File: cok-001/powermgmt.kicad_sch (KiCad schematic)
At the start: 39 parts, among them J6004 +12V_MAIN, J6005 +5V_EVER, Q6001 FDQ7238AS, Q6002 FDQ7238AS, U6003 MB39A, U6008 NCP511SN18T1, U6011 NCP511, U6012 MM3141, U6014 MM1591, U6019 NCP511SN18T1, U6021 MM1591, U6022 MM1593

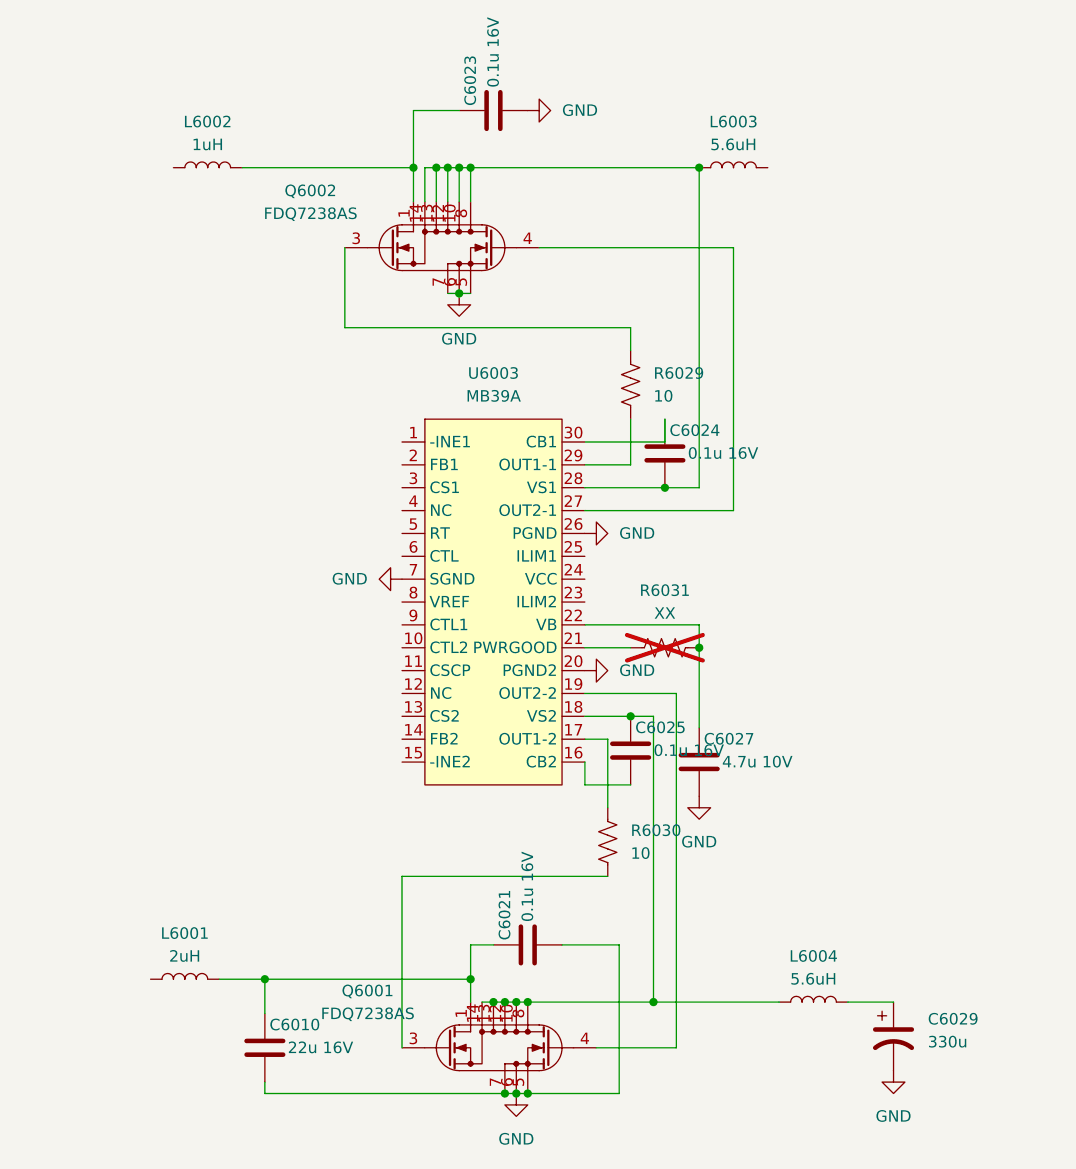
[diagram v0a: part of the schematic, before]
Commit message: update to 9
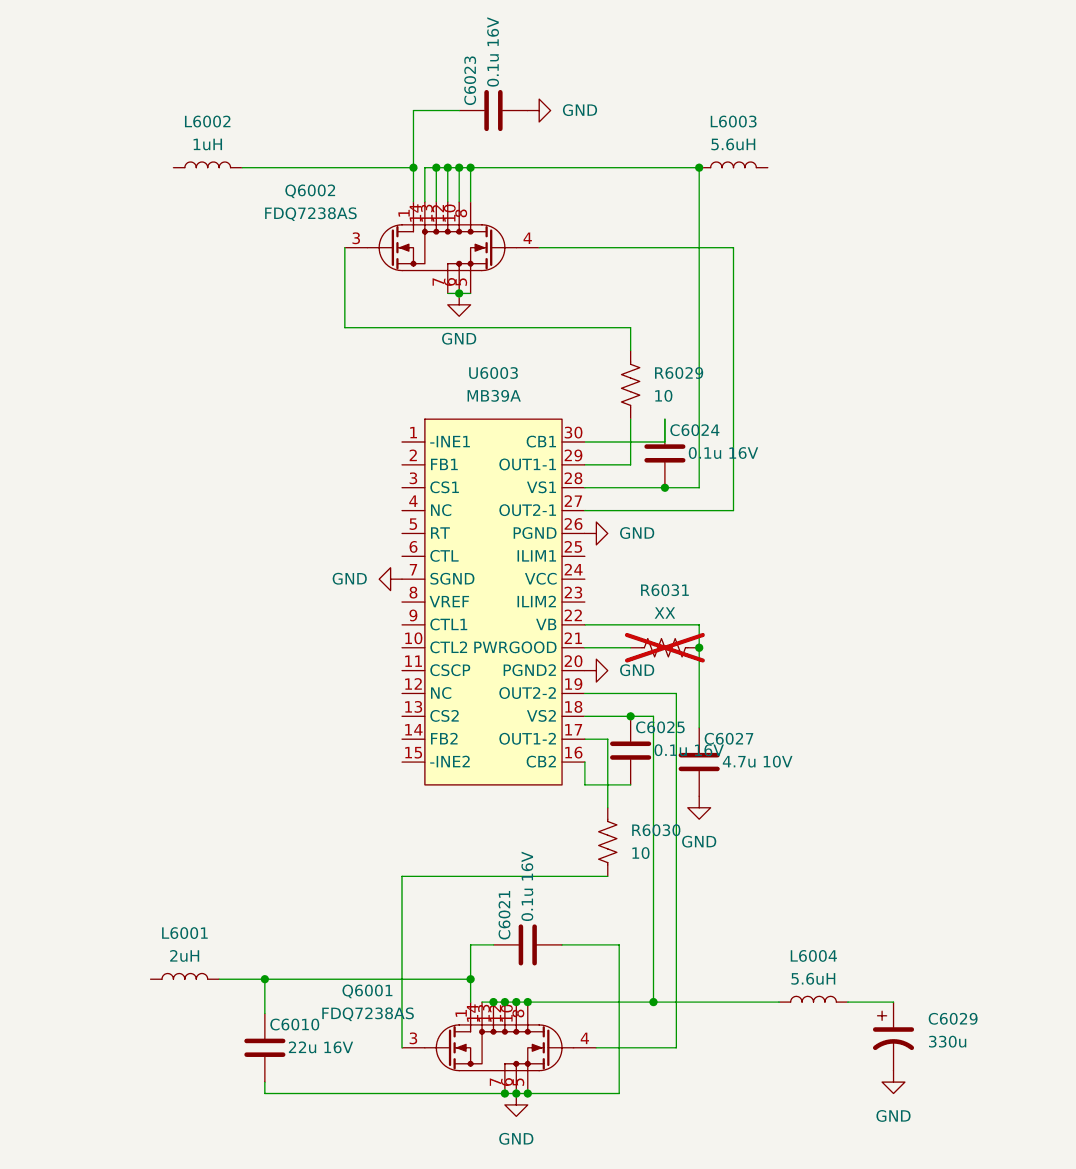
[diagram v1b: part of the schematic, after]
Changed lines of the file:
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@@
 (kicad_sch
-	(version 20231120)
+	(version 20250114)
 	(generator "eeschema")
-	(generator_version "8.0")
+	(generator_version "9.0")
 	(paper "A4")
 	(junction
